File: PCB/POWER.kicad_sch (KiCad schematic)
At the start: 24 parts, among them J2 Jack-DC, J3 Conn_01x07, Q10 P_Mosfet, U1 AMS1117, U1 XL1509

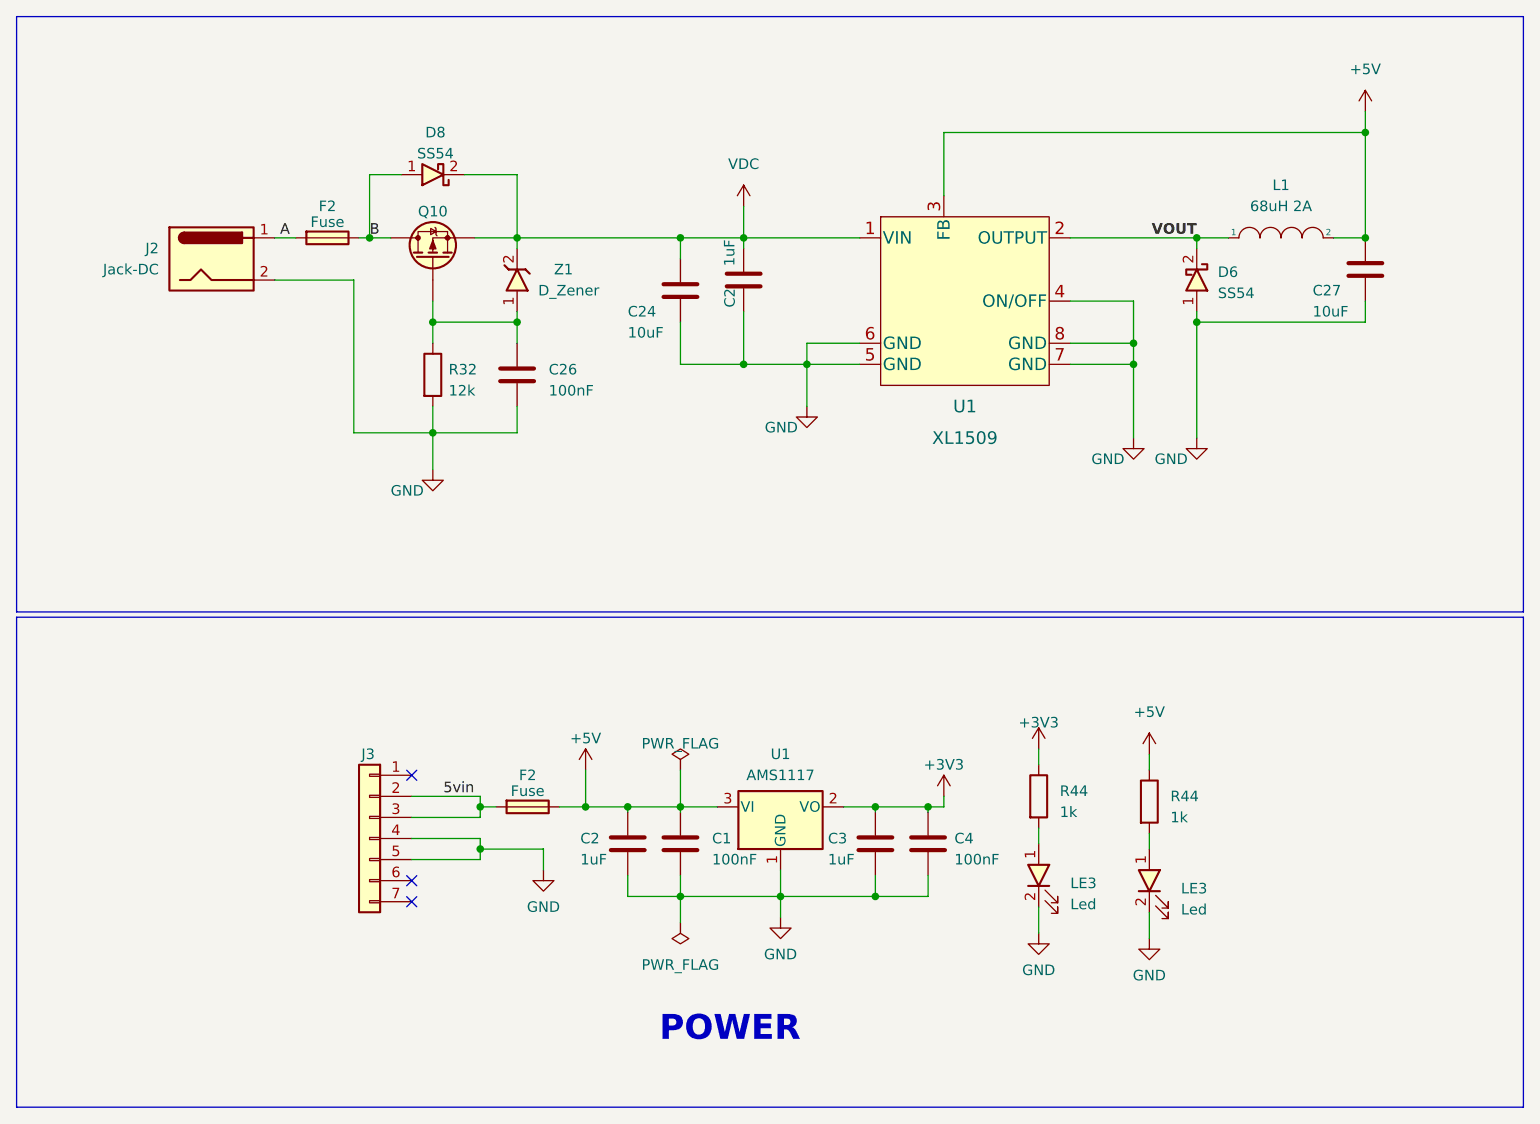
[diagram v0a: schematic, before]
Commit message: raw placement
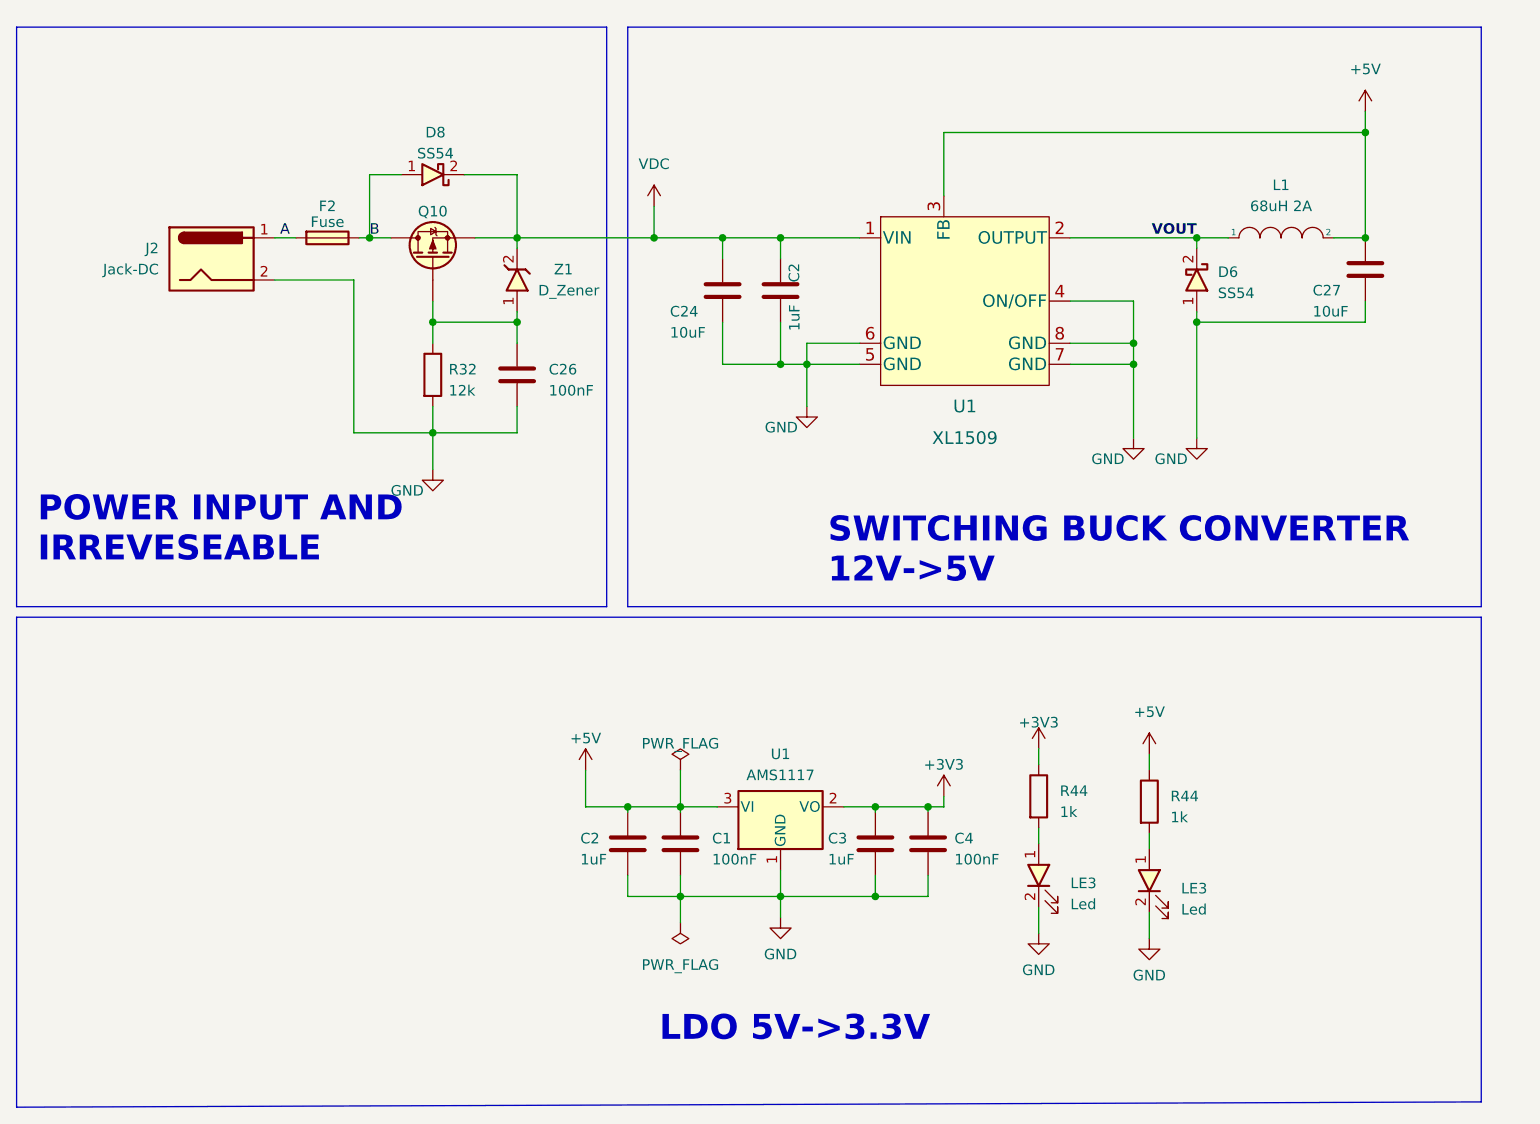
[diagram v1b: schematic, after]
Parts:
- removed F2: Fuse, IVS_FOOTPRINTS:Fuse_1812_4532Metric, symbol IVS_SYMBOLS:Fuse
- removed J3: Conn_01x07, IVS_FOOTPRINTS:Conn_XH-P2.54mm-7P, symbol Connector_Generic:Conn_01x07
- C2: footprint IVS_FOOTPRINTS:C_0603_1608Metric -> IVS_FOOTPRINTS:C_0603
- C27: footprint IVS_FOOTPRINTS:C_0805 -> IVS_FOOTPRINTS:CP_EIA-3528-15_AVX-H
- Z1: footprint (none) -> IVS_FOOTPRINTS:D_MiniMELF
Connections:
- net GND: now also C2.2; no longer C2.1
- net VDC: now also C2.1; no longer C2.2
- no-connect marks 3 -> 0
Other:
- note added: "LDO 5V->3.3V"
- note added: "POWER INPUT AND IRREVESEABLE"
- note added: "SWITCHING BUCK CONVERTER 12V->5V"
- note removed: "POWER"
- moved on the sheet: C2, C24
